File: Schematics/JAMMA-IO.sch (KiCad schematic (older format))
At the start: 107 parts, among them CN1 B6P-VH, CN2 VGA-DSUB15, CN3 BS4PSHF1AA, CN5 B12PSHF1A, U1 KONAMI-058232, U2 ADC0834

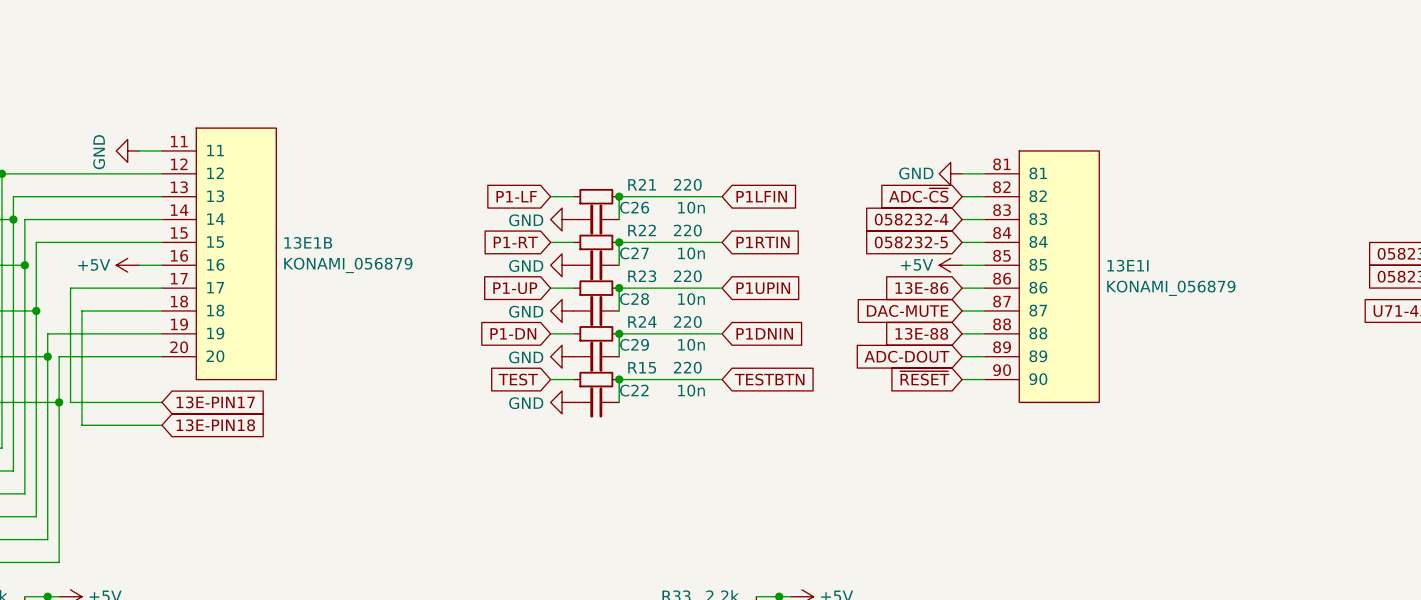
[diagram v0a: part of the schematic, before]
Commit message: 573 specific mostly mapped
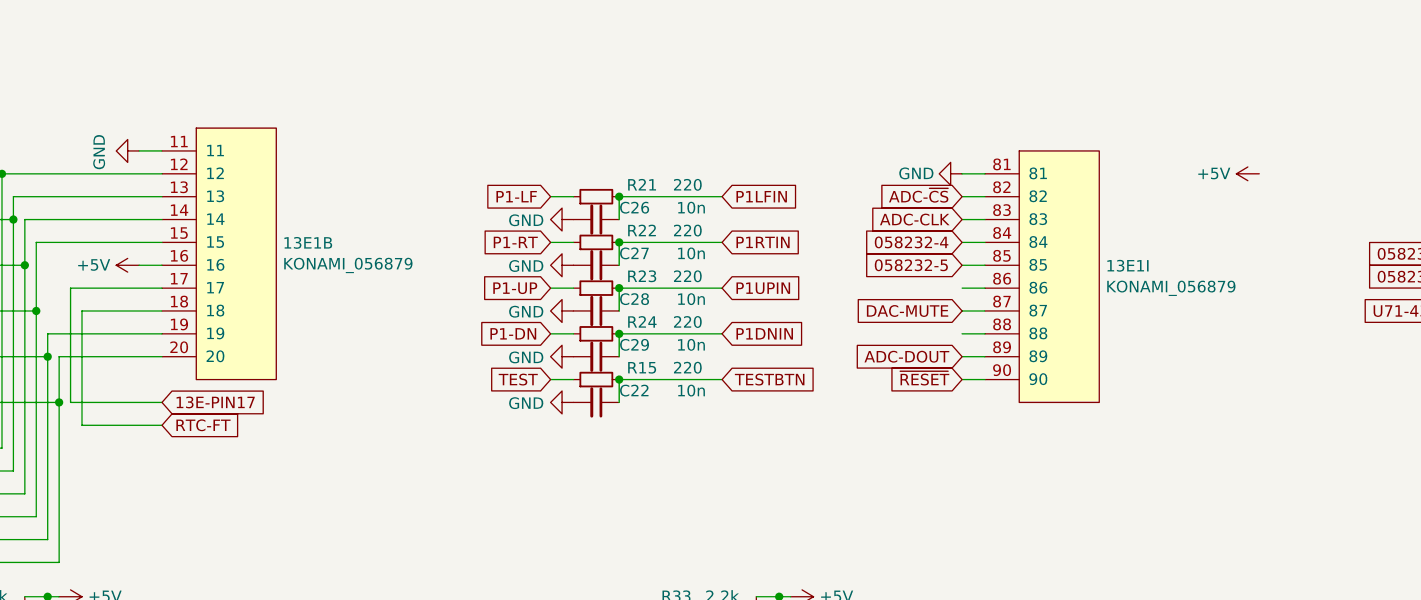
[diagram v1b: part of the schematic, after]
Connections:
- net +5V: no longer 13E1.85
- net 058232-4: now also 13E1.84; no longer 13E1.83
- net 058232-5: now also 13E1.85; no longer 13E1.84
- net ADC-CLK: now also 13E1.83
- net 13E-86: no longer names the net of 13E1.86
- net 13E-88: no longer names the net of 13E1.88
- net 13E-PIN18 renamed RTC-FT
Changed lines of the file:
@@
 13E-PIN17
 Text GLabel 8100 4250 2    50   Input ~ 0
-13E-PIN18
+RTC-FT
 Wire Wire Line
 	8100 3650 7700 3650
@@
 ADC-~CS
 Text GLabel 11600 3350 0    50   Input ~ 0
+ADC-CLK
+Text GLabel 11600 3450 0    50   Input ~ 0
 058232-4
-Text GLabel 11600 3450 0    50   Input ~ 0
-058232-5
 $Comp
 L power:+5V #PWR?
 U 1 1 620037C6
-P 11600 3550
+P 12900 3150
 AR Path="/620037C6" Ref="#PWR?"  Part="1"
 AR Path="/63647603/620037C6" Ref="#PWR0105"  Part="1"
-F 0 "#PWR0105" H 11600 3400 50  0001 C CNN
-F 1 "+5V" V 11600 3750 50  0000 C CNN
-F 2 "" H 11600 3550 50  0001 C CNN
-F 3 "" H 11600 3550 50  0001 C CNN
-	1    11600 3550
+F 0 "#PWR0105" H 12900 3000 50  0001 C CNN
+F 1 "+5V" V 12900 3350 50  0000 C CNN
+F 2 "" H 12900 3150 50  0001 C CNN
+F 3 "" H 12900 3150 50  0001 C CNN
+	1    12900 3150
 	0    -1   -1   0
 $EndComp
@@
 	0    1    1    0
 $EndComp
-Text GLabel 11600 3650 0    50   Input ~ 0
-13E-86
 Text GLabel 11600 3750 0    50   Input ~ 0
 DAC-MUTE
-Text GLabel 11600 3850 0    50   Input ~ 0
-13E-88
 Text GLabel 11600 4050 0    50   Input ~ 0
 ~RESET
@@
 Wire Wire Line
 	13700 3750 13900 3750
+Text GLabel 11600 3550 0    50   Input ~ 0
+058232-5
 $EndSCHEMATC
